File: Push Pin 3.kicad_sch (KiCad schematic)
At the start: 34 parts, among them J1 Screw_Terminal_01x02, J2 Screw_Terminal_01x02, J3 Screw_Terminal_01x02, J4 Screw_Terminal_01x02, J5 Screw_Terminal_01x02, J6 Screw_Terminal_01x02, J7 Screw_Terminal_01x02, Q1 NTR4101PT1G, Q2 NTR4101PT1G, Q3 NTR4101PT1G, SW4 SW_DPDT_x2, SW5 SW_DPDT_x2, SW6 SW_DPDT_x2, U2 LDO_4v2-MIC5209-4.2YS-TR

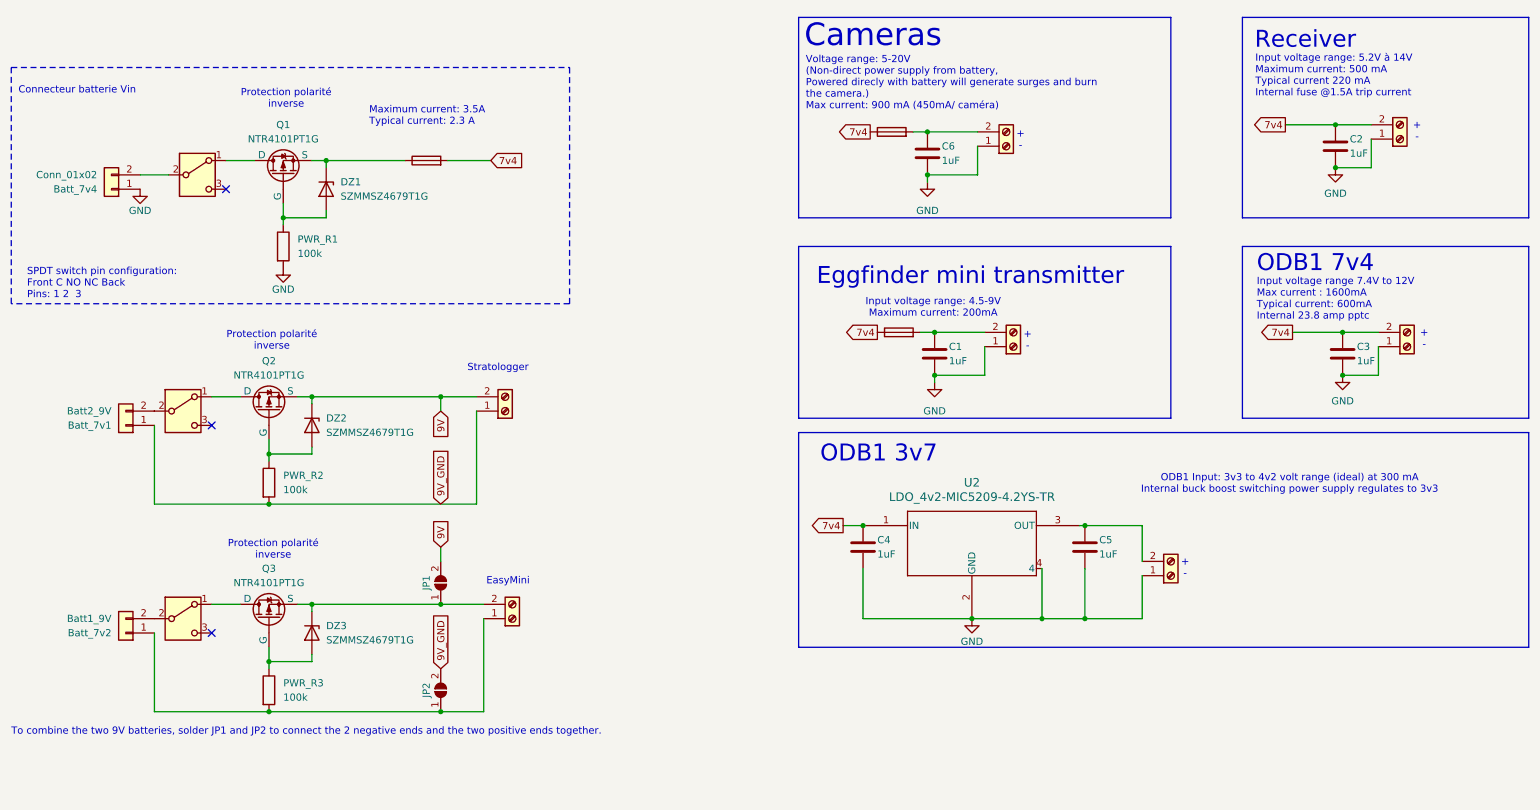
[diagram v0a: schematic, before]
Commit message: Plus beau
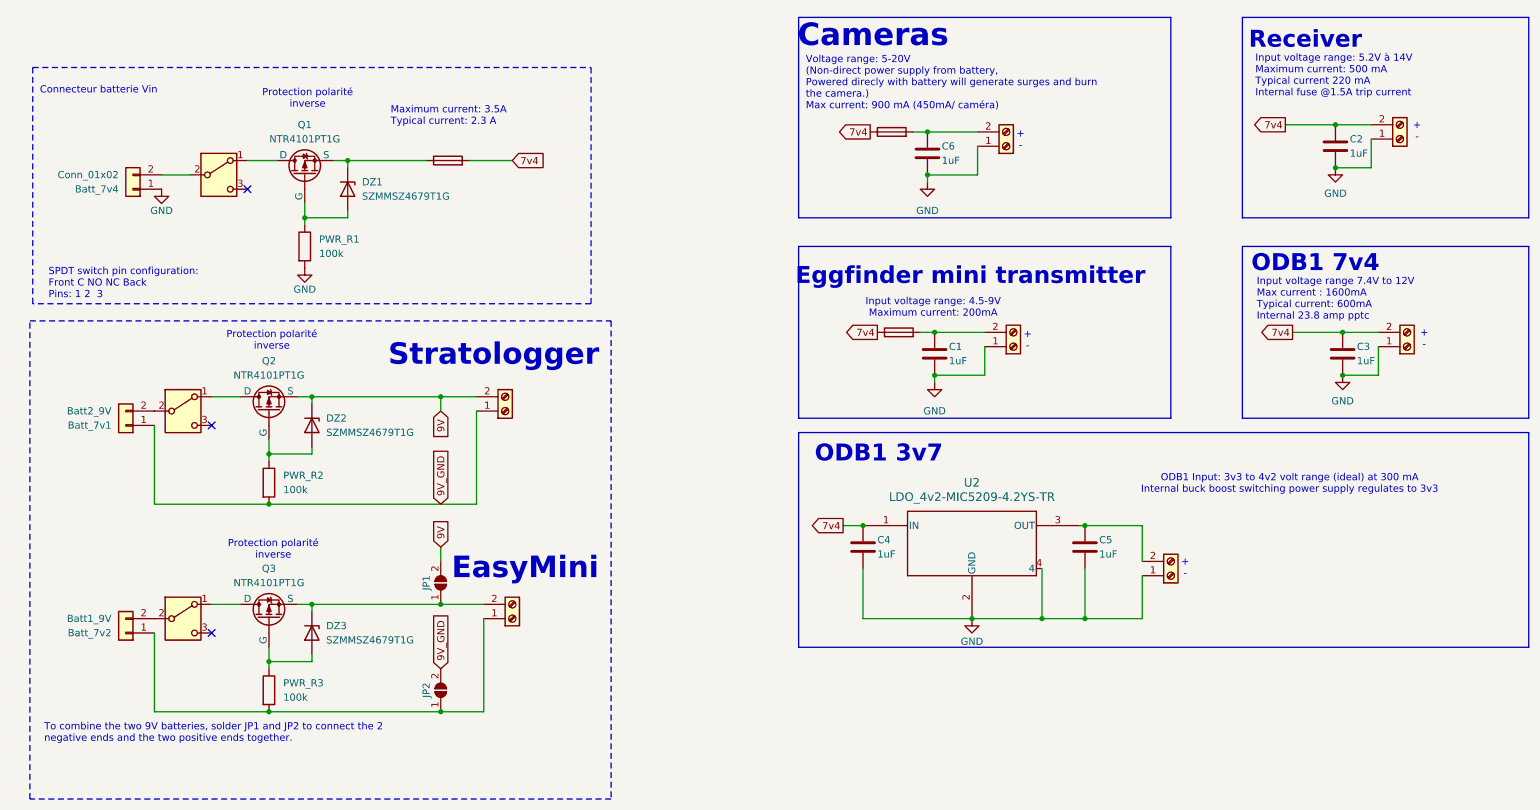
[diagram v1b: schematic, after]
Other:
- moved on the sheet: Batt_7v4, DZ1, PWR_R1, Q1
